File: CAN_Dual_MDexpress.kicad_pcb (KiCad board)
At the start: 2 copper layers, 84.4 x 82.5 mm, 140 parts, among them IC1 SI8650AB-B-IS1, IC2 AP7381-50SA-7, IC3 A3921KLPTR-T, IC4 SI8650AB-B-IS1, IC5 A3921KLPTR-T, J1 Conn_01x03, J2 Conn_01x05, J3 Bus_mechaken_PCIexpress_x16_1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, J4 Conn_01x02, J5 Conn_01x02, Q1 NVMFD5C446NT1G, Q2 NVMFD5C446NT1G, Q3 NVMFD5C446NT1G, Q4 NVMFD5C446NT1G, U1 LDL1117S33R_SOT223-4, U2 STM32F042K6Tx, U3 MCP2562-E-SN

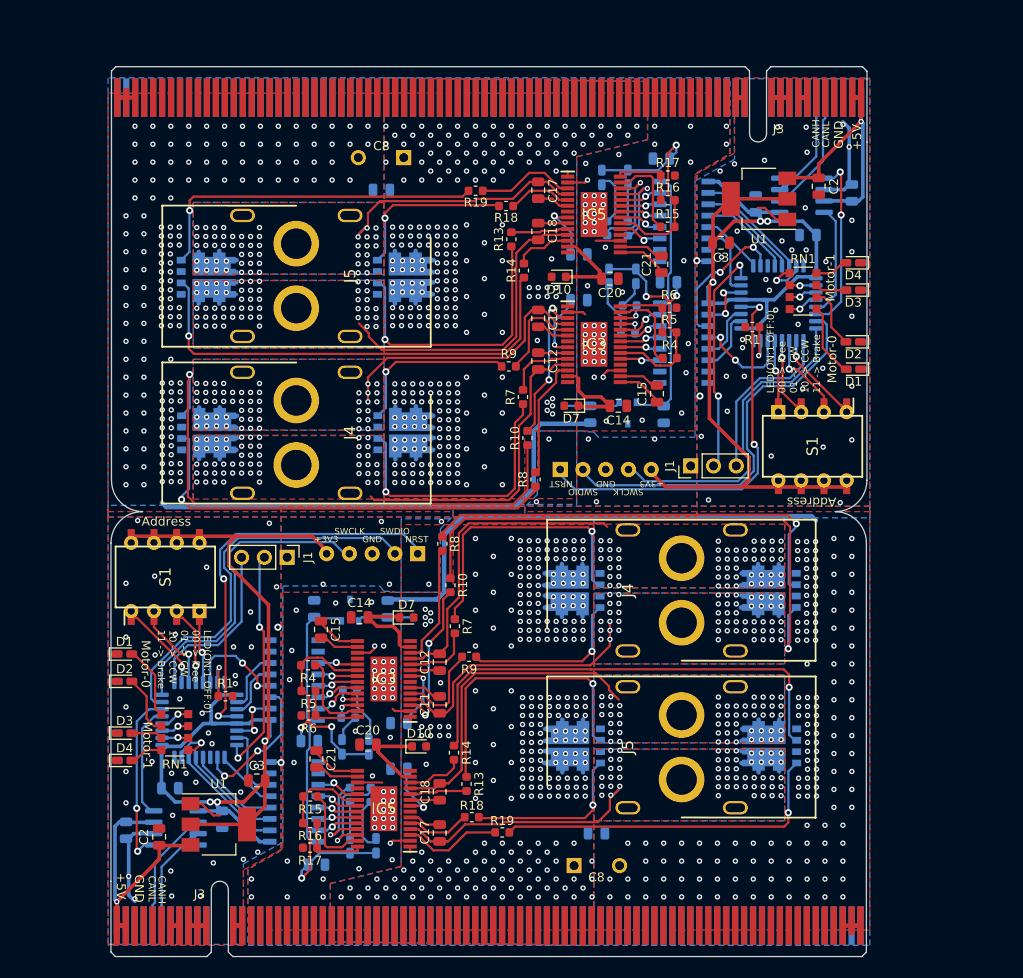
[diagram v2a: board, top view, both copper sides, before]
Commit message: clean
ガーバーデータを出力
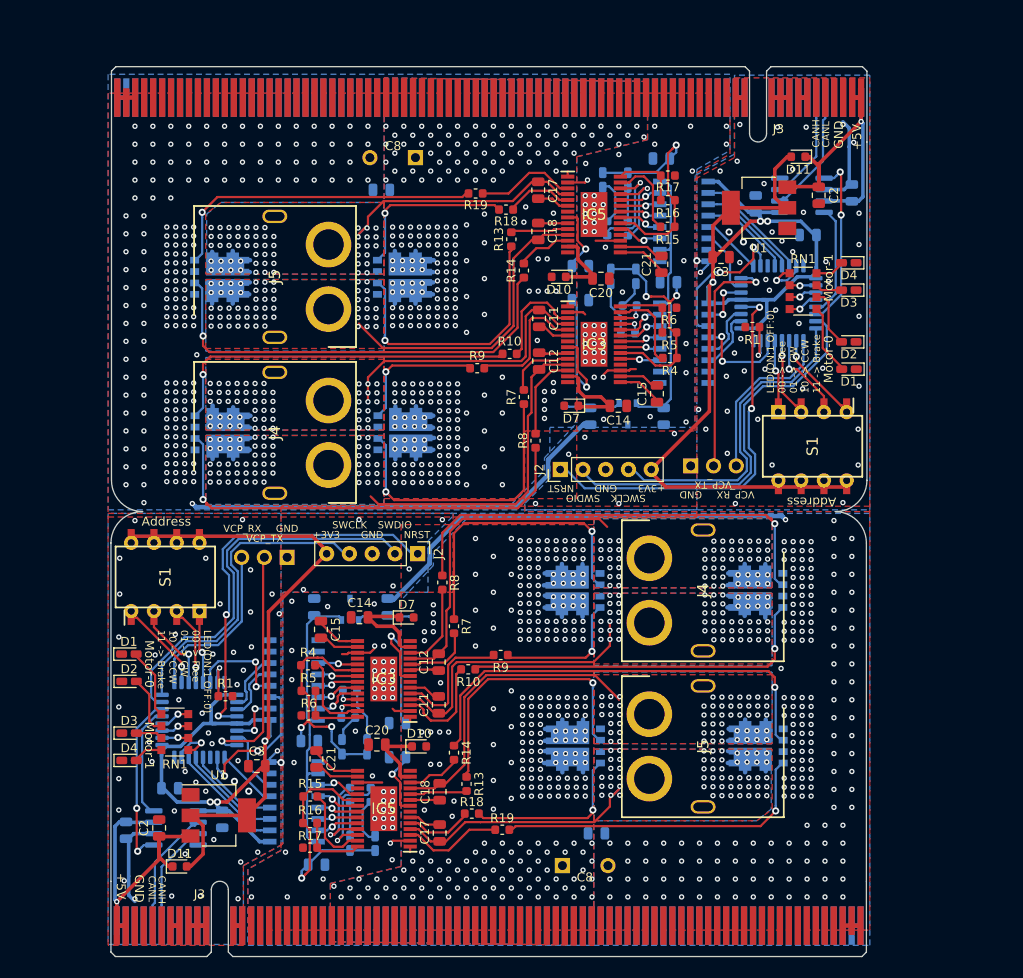
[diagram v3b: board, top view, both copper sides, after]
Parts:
- added D11: D_Schottky, Diode_SMD:D_0603_1608Metric, F.Cu at (192.0, 50.4)
- added D11: D_Schottky, Diode_SMD:D_0603_1608Metric, F.Cu at (123.0, 129.6)
- J1 (x2): value Conn_01x03 -> VCP; moved to B.Cu
- J2 (x2): value Conn_01x05 -> Conthrough; moved to F.Cu
- J4 (x2), J5 (x2): value Conn_01x02 -> XT60PW-M; footprint XT60:XT60PW_Reversible -> XT60:XT60PW
- RN1 (x2): value 2.2k -> 4.7k
- S2 (x2): footprint Package_DIP:DIP-8_W7.62mm -> Button_Switch_THT:SW_DIP_SPSTx04_Slide_9.78x12.34mm_W7.62mm_P2.54mm
- moved R10 9.60 mm to (159.8, 72.4), turned to 0 degrees
- moved R10 9.60 mm to (155.2, 107.6), turned to 180 degrees
- moved R8 4.32 mm to (162.7, 82.1)
- moved R8 4.32 mm to (152.3, 97.9)
- moved J5 3.60 mm to (139.6, 63.8), turned to 90 degrees
- moved J5 3.60 mm to (175.4, 116.2), turned to 270 degrees
- moved J4 3.60 mm to (139.6, 81.2), turned to 90 degrees
- moved J4 3.60 mm to (175.4, 98.8), turned to 270 degrees
- moved R9 3.53 mm to (156.2, 74.0)
- moved R9 3.53 mm to (158.8, 106.0)
- moved C3 1.60 mm to (183.4, 61.6)
- moved C3 1.60 mm to (131.6, 118.4)
- moved Q4 1.50 mm to (127.2, 63.9)
- moved Q4 1.50 mm to (187.8, 116.2)
- moved Q2 1.50 mm to (127.2, 81.2)
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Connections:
- net DIP_SW_1 renamed /DIP_SW1
- net DIP_SW_2 renamed /DIP_SW2
- net DIP_SW_3 renamed /DIP_SW3
- net DIP_SW_4 renamed /DIP_SW4
- net MD_FF1_0 renamed Net-(IC3-Pad25)
- net MD_FF1_1 renamed Net-(IC5-Pad26)
- net MD_FF2_0 renamed Net-(IC3-Pad26)
- net MD_FF2_1 renamed Net-(IC5-Pad25)
- net VREG_0 renamed /VREG_0
- net VREG_1 renamed /VREG_1
- IC1 pad 10: Net-(IC1-Pad10) -> MD_3V3 (x2)
- IC4 pad 10: Net-(IC4-Pad10) -> MD_3V3 (x2)
- J4 pad 1: SB_0 -> SA_0 (x2)
- J4 pad 2: SA_0 -> SB_0 (x2)
- J5 pad 1: SB_1 -> SA_1 (x2)
- J5 pad 2: SA_1 -> SB_1 (x2)
- R15 pad 1: Net-(IC5-Pad27) -> V5_1 (x2)
- R15 pad 2: V5_1 -> Net-(IC5-Pad27) (x2)
- R16 pad 1: Net-(IC5-Pad28) -> V5_1 (x2)
- R16 pad 2: V5_1 -> Net-(IC5-Pad28) (x2)
- R4 pad 1: Net-(IC3-Pad27) -> V5_0 (x2)
- R4 pad 2: V5_0 -> Net-(IC3-Pad27) (x2)
- R5 pad 1: Net-(IC3-Pad28) -> V5_0 (x2)
- R5 pad 2: V5_0 -> Net-(IC3-Pad28) (x2)
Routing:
- net Net-(Q2-Pad4): track 125.2 -> 79.9 mm
- net /VREG_0: track 13.4 -> 32.5 mm
- net +3V3: track 239.9 -> 252.9 mm
- net +5V: track 65.2 -> 76.5 mm
- net GLB_0: track 34.3 -> 23.1 mm, vias 4 -> 0
- net GNDPWR: track 135.8 -> 126.6 mm, vias 392 -> 444
- net GHB_0: track 21.3 -> 29.3 mm
- net GLA_0: track 26.9 -> 19.1 mm
- net MD_3V3: track 65.4 -> 73.0 mm
- net Net-(Q1-Pad4): track 37.7 -> 30.6 mm
- net Net-(Q4-Pad2): track 105.2 -> 99.7 mm
- net Net-(Q4-Pad4): track 77.2 -> 72.7 mm
- net GND: track 32.3 -> 27.8 mm, vias 86 -> 100
- net VCP_TX: track 51.2 -> 54.6 mm, vias 4 -> 2
- net SA_1: track 74.0 -> 71.2 mm, vias 104 -> 110
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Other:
- board text added: "isolator GND NC PHASE SR PWML PWMH RESET +3V3"
- board text removed: "Conthrough"
